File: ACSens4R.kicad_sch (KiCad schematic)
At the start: 5 parts, among them U2 PC817

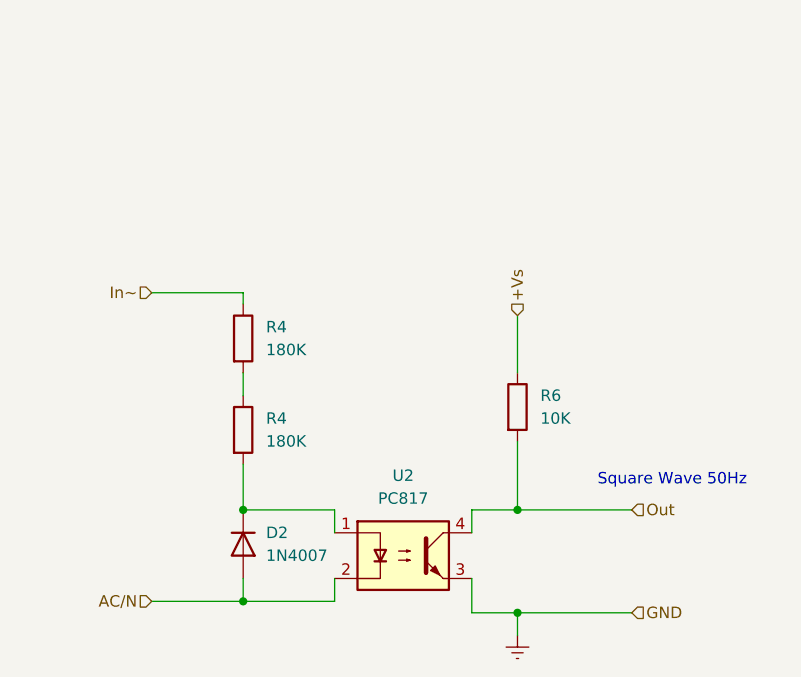
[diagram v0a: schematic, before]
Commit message: Version 1.1
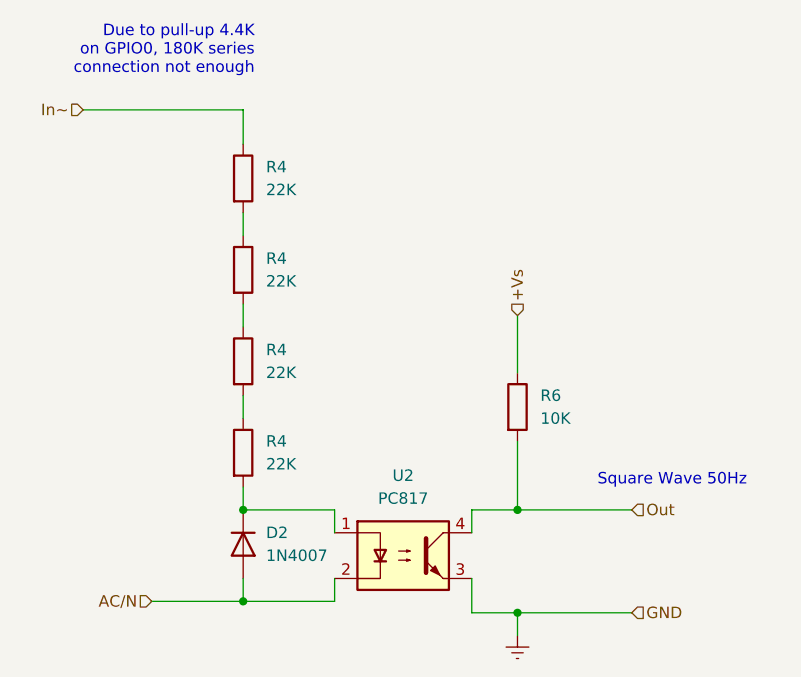
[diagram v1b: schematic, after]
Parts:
- removed R4 (x2): 180K, Resistor_SMD:R_0805_2012Metric_Pad1.20x1.40mm_HandSolder, symbol Device:R
- added R4 (x4): 22K, Resistor_SMD:R_1206_3216Metric_Pad1.30x1.75mm_HandSolder, symbol Device:R
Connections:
- net In~: now also R4.1
- net at D2.1 (K), U2.1: now also R4.2
- new net: R4.1, R4.2 (x3)
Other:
- note added: "Due to pull-up 4.4K on GPIO0, 180K series connection not enough"
